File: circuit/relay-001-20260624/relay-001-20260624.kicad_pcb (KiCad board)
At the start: 2 copper layers, 169 x 126.3 mm, 15 parts, among them J1 Conn_01x03_Pin, J10 Conn_01x02_Pin, J11 Conn_01x02_Pin, J12 Conn_01x02_Pin, J13 Conn_01x02_Pin, J14 Conn_01x02_Pin, J15 Conn_01x02_Pin, J2 Conn_02x05_Odd_Even, J3 Conn_02x08_Odd_Even, J4 Conn_02x09_Odd_Even, J5 Conn_01x02_Pin, J6 Conn_01x02_Pin, J7 Conn_01x02_Pin, J8 Conn_01x02_Pin, J9 Conn_01x02_Pin

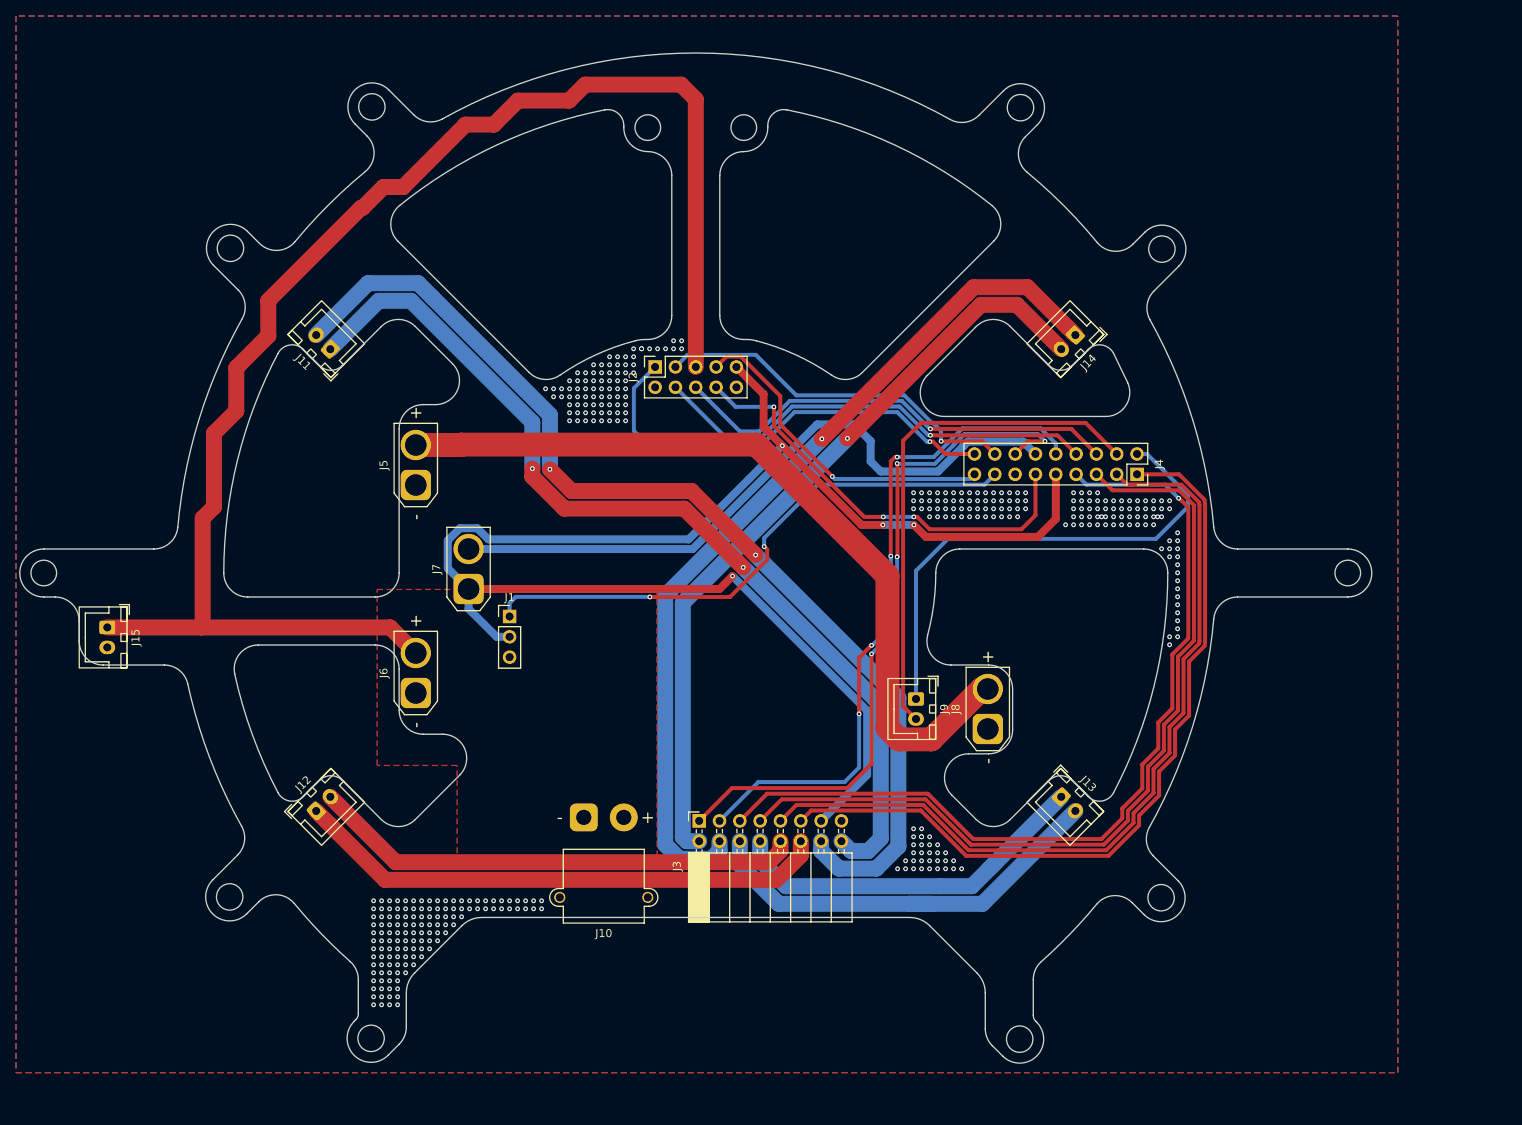
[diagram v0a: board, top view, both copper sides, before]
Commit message: Update 供給基板の3DファイルとPCBを出力
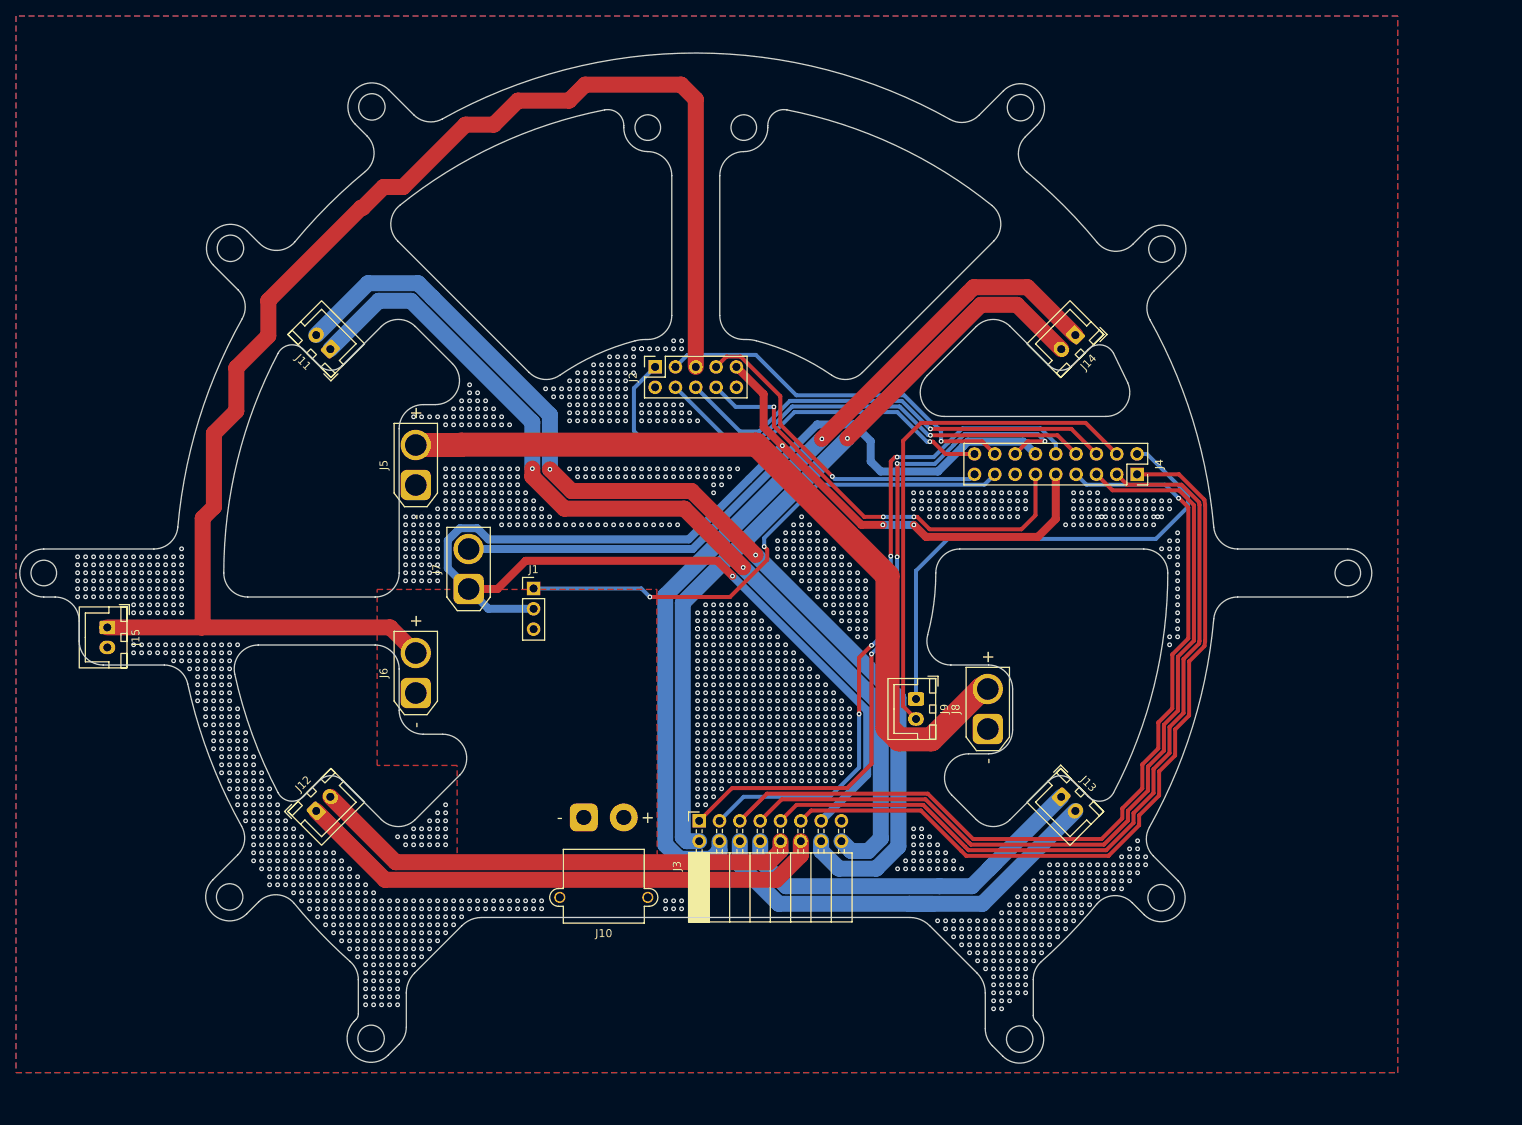
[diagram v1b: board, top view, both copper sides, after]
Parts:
- moved J1 4.61 mm to (98.0, 93.5)
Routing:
- net Dribbler_{Back}: track 71.1 -> 66.6 mm
- net +3.3V: track 195.3 -> 197.0 mm
- net GND: vias 373 -> 1699

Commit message: Update 供給基板のPCBが完成した
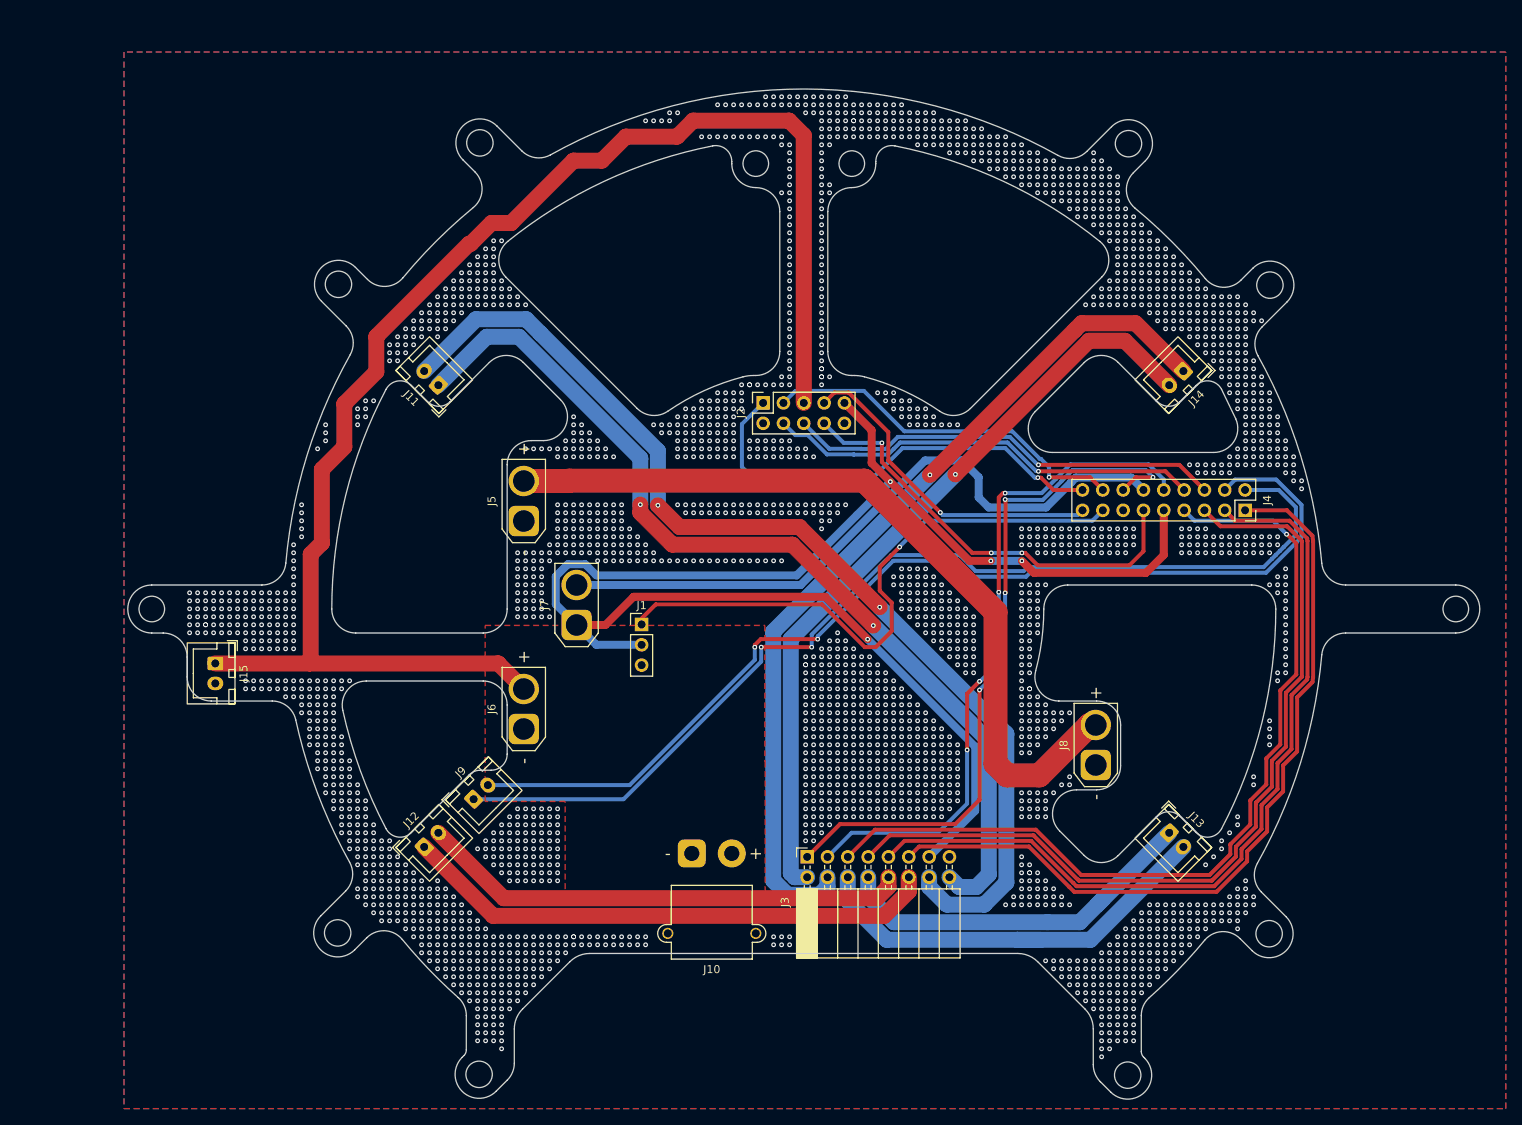
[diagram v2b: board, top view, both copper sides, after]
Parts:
- moved J9 56.7 mm to (90.5, 119.8), turned to 45 degrees
- moved J1 14.2 mm to (111.5, 98.0)
- moved J10 14.2 mm to (117.8, 126.6)
- moved J11 14.2 mm to (86.1, 68.0)
- moved J12 14.2 mm to (84.3, 125.8)
- moved J13 14.2 mm to (177.5, 124.0)
- moved J15 14.2 mm to (58.2, 102.8)
- moved J2 14.2 mm to (126.7, 70.3)
- moved J3 14.2 mm to (132.2, 127.0)
- moved J4 14.2 mm to (186.9, 83.7)
- moved J5 14.2 mm to (96.8, 85.0)
- moved J6 14.2 mm to (96.8, 111.0)
- moved J7 14.2 mm to (103.4, 98.0)
- moved J8 14.2 mm to (168.3, 115.5)
- moved J14 14.2 mm to (179.2, 66.3)
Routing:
- net RX_{teensy}-TX_{Arduino}-5V: track 64.7 -> 133.0 mm, vias 0 -> 2
- net TX_{teensy}-RX_{Arduino}-5V: track 63.3 -> 130.8 mm, vias 0 -> 2
- net Dribbler_{Back}: track 66.6 -> 75.3 mm, vias 2 -> 1
- net PH_{Dribbler-Front}: track 56.7 -> 54.8 mm
- net EN_{Dribbler-Front}: track 56.7 -> 54.8 mm
- net GND: vias 1699 -> 2549
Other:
- outline, holes or cut-outs redrawn
